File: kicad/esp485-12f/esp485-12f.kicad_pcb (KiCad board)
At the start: 2 copper layers, 33 x 20.3 mm, 19 parts, among them J1 Conn_01x04, SW1 SW_Push, SW2 SW_Push, U1 MAX3485, U2 ESP-12F, U3 AMS1117-3.3

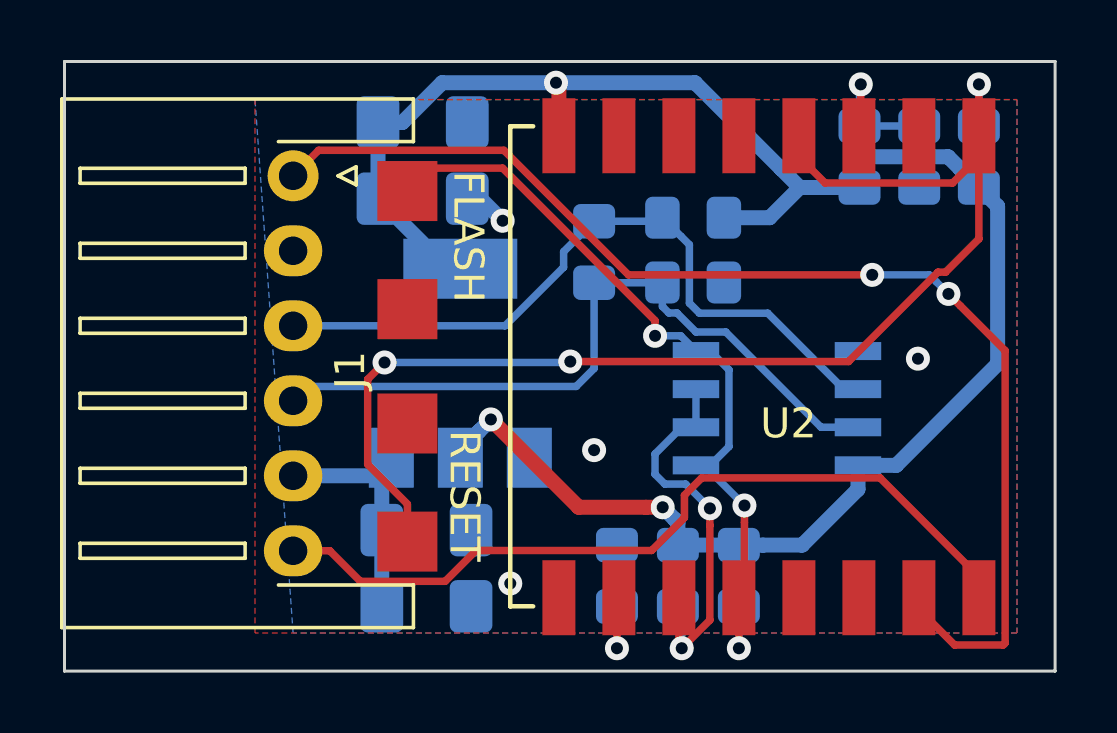
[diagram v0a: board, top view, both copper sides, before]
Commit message: remove switches
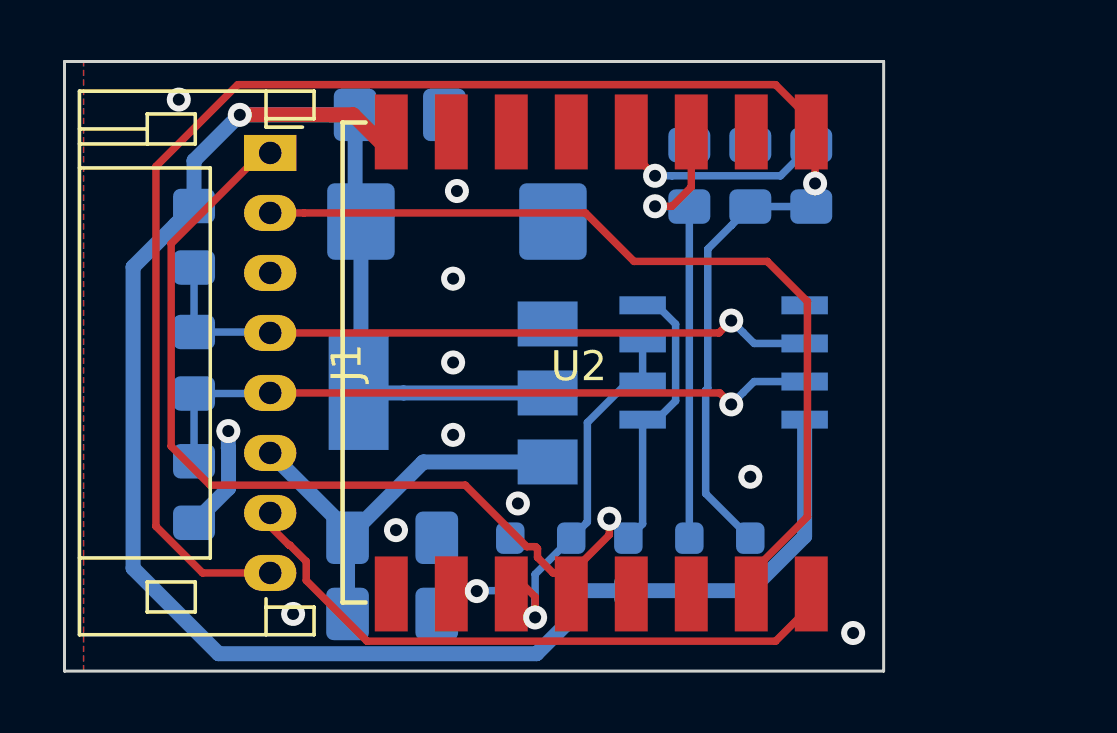
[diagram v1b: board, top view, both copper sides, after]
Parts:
- removed SW1, SW2: SW_Push, tact:tactile_switch_smd_4x3mm_2p
- added C6: C, Capacitor_SMD:C_0805_2012Metric_Pad1.15x1.40mm_HandSolder, B.Cu at (129.5, 111.8)
- added R6: 1K, Resistor_SMD:R_0805_2012Metric_Pad1.15x1.40mm_HandSolder, B.Cu at (131.6, 111.8)
- C3: footprint Capacitor_SMD:C_1206_3216Metric_Pad1.42x1.75mm_HandSolder -> Capacitor_Tantalum_SMD:CP_EIA-7343-15_Kemet-W_Pad2.25x2.55mm_HandSolder
- J1: value Conn_01x04 -> Conn_01x08; footprint Connector_JST:JST_XH_S06B-XH-A-1_1x06_P2.50mm_Horizontal -> Connector_JST:JST_PH_S8B-PH-K_1x08_P2.00mm_Horizontal
- R1, R2, R3, R7, R9: footprint Resistor_SMD:R_0805_2012Metric_Pad1.15x1.40mm_HandSolder -> Resistor_SMD:R_0603_1608Metric_Pad1.05x0.95mm_HandSolder
- moved R5 18.0 mm to (111.0, 122.3), turned to 270 degrees
- moved R4 16.6 mm to (111.0, 113.8), turned to 270 degrees
- moved R3 15.6 mm to (129.5, 124.7)
- moved R1 14.7 mm to (127.5, 124.7)
- moved R10 13.8 mm to (111.0, 118.0)
- moved C5 7.69 mm to (127.5, 111.8), turned to 90 degrees
- moved U2 5.59 mm to (131.6, 111.0)
- moved R7 3.70 mm to (125.5, 124.7), turned to 90 degrees
- moved R2 3.58 mm to (123.6, 124.7), turned to 270 degrees
- moved R9 3.58 mm to (121.5, 124.7)
- moved U1 2.34 mm to (128.7, 118.0)
- moved C3 1.37 mm to (119.8, 113.3)
- moved C1 1.17 mm to (117.6, 123.8)
- moved C2 1.17 mm to (117.6, 126.4)
- moved J1 1.08 mm to (113.5, 111.0)
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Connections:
- J1 pad 1: /RXD -> /IO0
- J1 pad 2: GND -> /RXD
- J1 pad 3: /A -> GND
- J1 pad 4: /B -> /A
- J1 pad 5: VCC -> /B
- J1 pad 6: /TXD -> VCC
- U2 pad 13: (no net) -> Net-(U2-Pad13)
- U2 pad 14: (no net) -> Net-(U2-Pad14)
- U2 pad 2: (no net) -> Net-(U2-Pad2)
- U2 pad 4: /RESET -> Net-(R6-Pad1)
- U2 pad 5: (no net) -> Net-(U2-Pad5)
- U2 pad 6: (no net) -> Net-(U2-Pad6)
- U2 pad 7: (no net) -> Net-(U2-Pad7)
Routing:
- net /RESET: track 41.5 -> 57.2 mm, vias 3 -> 1
- net /IO0: track 26.9 -> 39.2 mm, vias 3 -> 1
- net /RXD: track 41.1 -> 29.0 mm, vias 2 -> 0
- net /EN: track 5.83 -> 14.8 mm
- net +3V3: track 64.9 -> 71.9 mm, vias 3 -> 1
- net Net-(R6-Pad1): track 0.00 -> 6.74 mm, vias 0 -> 1
- net VCC: track 8.61 -> 14.2 mm
- net /TXD: track 26.5 -> 22.0 mm
- net /IO2: track 14.9 -> 12.7 mm, vias 2 -> 1
- net GND: track 1.48 -> 3.54 mm, vias 4 -> 11
- net /IO15: track 3.80 -> 2.22 mm
- net /B: track 24.6 -> 23.1 mm, vias 0 -> 1
- net /A: track 24.1 -> 23.0 mm, vias 0 -> 1
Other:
- board size 33 x 20.3 mm -> 27.3 x 20.3 mm
- board text removed: "FLASH"
- board text removed: "RESET"
